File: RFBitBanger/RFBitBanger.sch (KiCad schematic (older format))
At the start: 174 parts, among them J1 POWER, J10 Conn_01x03, J11 SPEAKER, J12 Conn_Coaxial, J2 Barrel_Jack, J3 Conn_01x01, J4 Conn_01x01, J5 Conn_01x04, J6 Conn_01x01, J7 Conn_01x01, J9 ICSP, Q1 SS8050, Q2 SS9018, Q3 SS8050, Q4 S8050, Q5 SS8050, Q6 SS8050, Q7 SS8050, Q8 2N3906, Q9 SS8050, SW1 SW_Push, SW2 SW_Push, SW3 SW_Push, SW4 SW_Push, SW5 SW_Push, T1 Trifilar, T2 Trifilar, T3 Current, U1 ATMEGA328-PU, U2 LM7805_TO220, U3 LM386, U4 LM358, U5 LCD-016N002L, U6 SI5351A, Y1 16 MHz, Y2 7.023 MHz, Y3 27 MHz

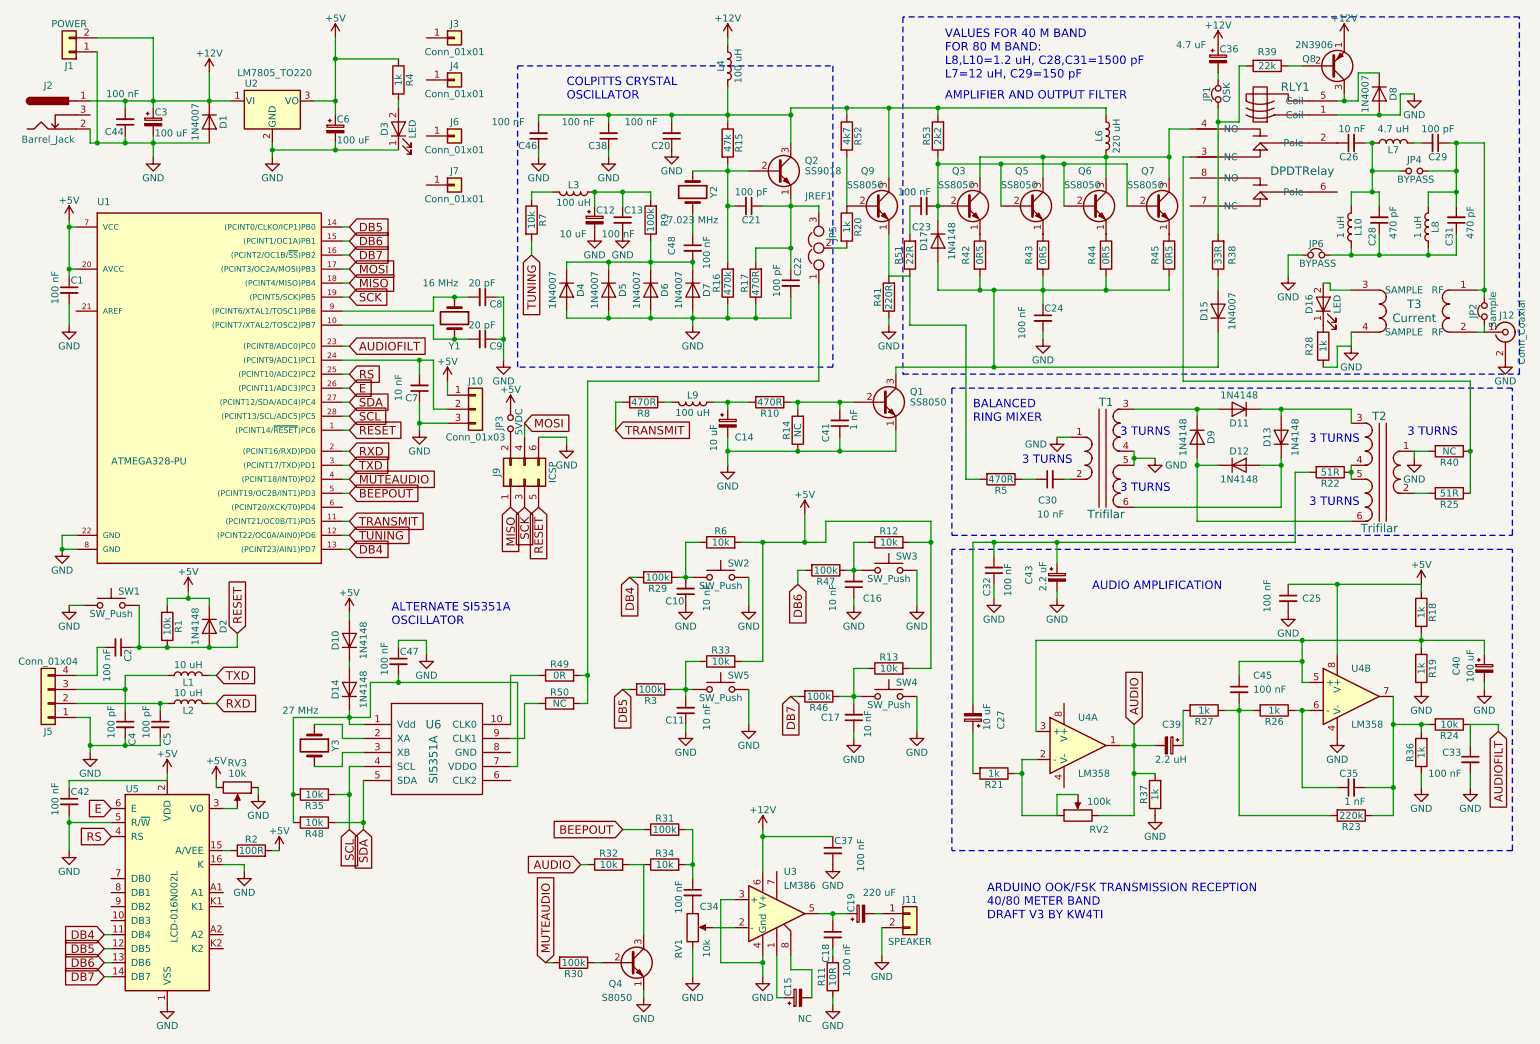
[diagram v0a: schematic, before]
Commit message: Completely remade board with common base input
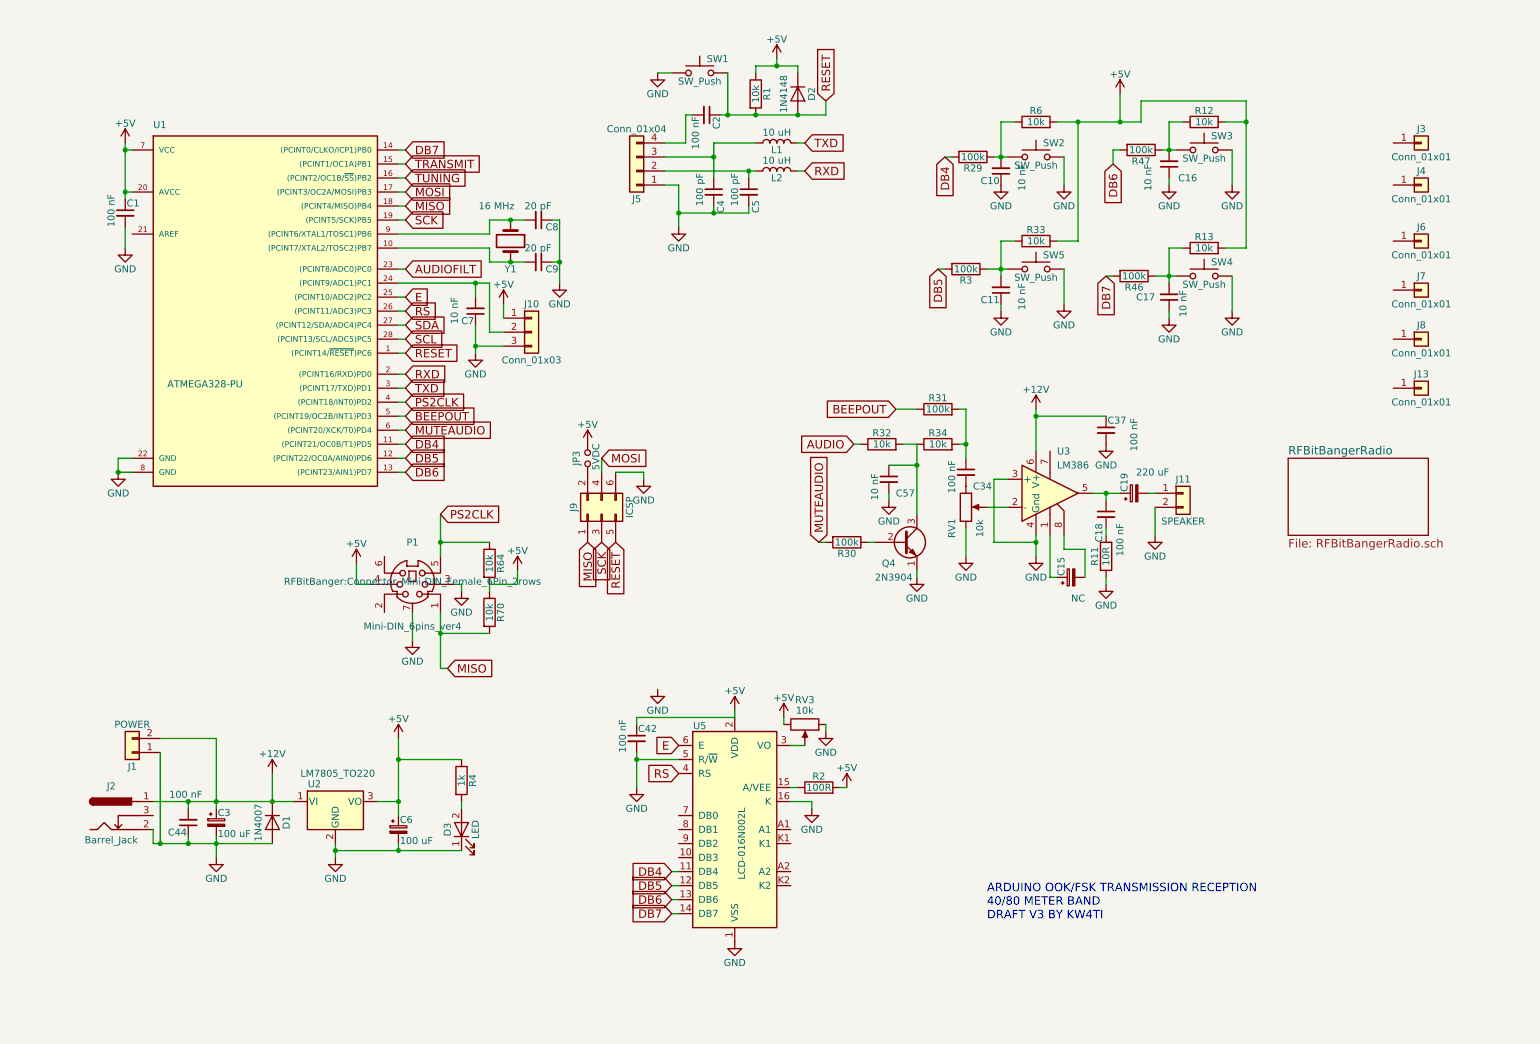
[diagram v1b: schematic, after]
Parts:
- removed C12, C14, C27: 10 uF, Capacitors_THT:CP_Radial_D5.0mm_P2.50mm, symbol CP_Small
- removed C13, C20, C23, C24, C25, C33, C38, C45, C46, C47, C48: 100 nF, Capacitors_THT:C_Disc_D5.0mm_W2.5mm_P2.50mm, symbol C_Small
- removed C21, C22, C29: 100 pF, Capacitors_THT:C_Disc_D5.0mm_W2.5mm_P5.00mm, symbol C_Small
- removed C26, C30: 10 nF, Capacitors_THT:C_Disc_D5.0mm_W2.5mm_P2.50mm, symbol C_Small
- removed C28, C31: 470 pF, Capacitors_THT:C_Disc_D5.0mm_W2.5mm_P5.00mm, symbol C_Small
- removed C32: 100 nF, Capacitors_THT:C_Disc_D5.0mm_W2.5mm_P5.00mm, symbol C_Small
- removed C35, C41: 1 nF, Capacitors_THT:C_Disc_D5.0mm_W2.5mm_P5.00mm, symbol C_Small
- removed C36: 4.7 uF, Capacitors_THT:CP_Radial_D5.0mm_P2.50mm, symbol CP_Small
- removed C39: 2.2 uH, Capacitors_THT:CP_Radial_D5.0mm_P2.50mm, symbol CP_Small
- removed C40: 100 uF, Capacitors_THT:CP_Radial_D5.0mm_P2.50mm, symbol CP_Small
- removed C43: 2.2 uF, Capacitors_THT:CP_Radial_D5.0mm_P2.50mm, symbol CP_Small
- removed D10, D11, D12, D13, D14, D17, D9: 1N4148, Diodes_THT:D_DO-35_SOD27_P7.62mm_Horizontal, symbol D
- removed D15, D4, D5, D6, D7, D8: 1N4007, Diodes_THT:D_DO-41_SOD81_P7.62mm_Horizontal, symbol D
- removed D16: LED, LEDs:LED_D3.0mm, symbol LED
- removed J12: Conn_Coaxial, RFBitBanger:bnc_90_1-1337543-0_pad_combo, symbol Conn_Coaxial
- removed JP1: QSK, Pin_Headers:Pin_Header_Straight_1x02_Pitch2.54mm, symbol Jumper_NC_Small
- removed JP2: Sample, Pin_Headers:Pin_Header_Straight_1x02_Pitch2.54mm, symbol Jumper_NC_Small
- removed JP4: BYPASS, Pin_Headers:Pin_Header_Straight_1x02_Pitch2.54mm, symbol Jumper_NO_Small
- removed JP5: JREF1, Pin_Headers:Pin_Header_Straight_1x03_Pitch2.54mm, symbol Jumper_NC_Dual
- removed JP6: BYPASS, Pin_Headers:Pin_Header_Straight_1x02_Pitch2.54mm, symbol Jumper_NC_Small
- removed L10, L8: 1 uH, Inductors_THT:L_Axial_L6.6mm_D2.7mm_P10.16mm_Horizontal_Vishay_IM-2, symbol L
- removed L3, L4, L9: 100 uH, Inductors_THT:L_Axial_L6.6mm_D2.7mm_P10.16mm_Horizontal_Vishay_IM-2, symbol L
- removed L6: 220 uH, Inductors_THT:L_Axial_L6.6mm_D2.7mm_P10.16mm_Horizontal_Vishay_IM-2, symbol L
- removed L7: 4.7 uH, Inductors_THT:L_Axial_L6.6mm_D2.7mm_P10.16mm_Horizontal_Vishay_IM-2, symbol L
- removed Q1, Q3, Q5, Q6, Q7, Q9: SS8050, TO_SOT_Packages_THT:TO-92_Inline_Wide, symbol 2N3904
- removed Q2: SS9018, TO_SOT_Packages_THT:TO-92_Inline_Wide, symbol 2N3904
- removed Q8: 2N3906, TO_SOT_Packages_THT:TO-92_Inline_Wide, symbol 2N3906
- removed R10, R17, R5, R8: 470R, Resistors_THT:R_Axial_DIN0207_L6.3mm_D2.5mm_P7.62mm_Horizontal, symbol R
- removed R14, R40, R50: NC, Resistors_THT:R_Axial_DIN0207_L6.3mm_D2.5mm_P7.62mm_Horizontal, symbol R
- removed R15: 47k, Resistors_THT:R_Axial_DIN0207_L6.3mm_D2.5mm_P7.62mm_Horizontal, symbol R
- removed R16: 470k, Resistors_THT:R_Axial_DIN0207_L6.3mm_D2.5mm_P7.62mm_Horizontal, symbol R
- removed R18, R19, R20, R21, R26, R27, R28, R36, R37: 1k, Resistors_THT:R_Axial_DIN0207_L6.3mm_D2.5mm_P7.62mm_Horizontal, symbol R
- removed R22, R25: 51R, Resistors_THT:R_Axial_DIN0207_L6.3mm_D2.5mm_P7.62mm_Horizontal, symbol R
- removed R23: 220k, Resistors_THT:R_Axial_DIN0207_L6.3mm_D2.5mm_P7.62mm_Horizontal, symbol R
- removed R24, R35, R48, R7: 10k, Resistors_THT:R_Axial_DIN0207_L6.3mm_D2.5mm_P7.62mm_Horizontal, symbol R
- removed R38: 33R, Resistors_THT:R_Axial_DIN0207_L6.3mm_D2.5mm_P7.62mm_Horizontal, symbol R
- removed R39: 22k, Resistors_THT:R_Axial_DIN0207_L6.3mm_D2.5mm_P7.62mm_Horizontal, symbol R
- removed R41: 220R, Resistors_THT:R_Axial_DIN0207_L6.3mm_D2.5mm_P7.62mm_Horizontal, symbol R
- removed R42, R43, R44, R45: 0R5, Resistors_THT:R_Axial_DIN0207_L6.3mm_D2.5mm_P7.62mm_Horizontal, symbol R
- removed R49: 0R, Resistors_THT:R_Axial_DIN0207_L6.3mm_D2.5mm_P7.62mm_Horizontal, symbol R
- removed R51: 22R, Resistors_THT:R_Axial_DIN0207_L6.3mm_D2.5mm_P7.62mm_Horizontal, symbol R
- removed R52: 4k7, Resistors_THT:R_Axial_DIN0207_L6.3mm_D2.5mm_P7.62mm_Horizontal, symbol R
- removed R53: 2k2, Resistors_THT:R_Axial_DIN0207_L6.3mm_D2.5mm_P7.62mm_Horizontal, symbol R
- removed R9: 100k, Resistors_THT:R_Axial_DIN0207_L6.3mm_D2.5mm_P7.62mm_Horizontal, symbol R
- removed RLY1: DPDTRelay, RFBitBanger:G2VRelay, symbol DPDTRelay
- removed RV2: 100k, Potentiometers:Potentiometer_WirePads, symbol POT
- removed T1, T2: Trifilar, RFBitBanger:TripleWindingTransformer, symbol TripleWindingTransformer
- removed T3: Current, RFBitBanger:SamplingTransformer, symbol Current
- removed U4: LM358, Housings_DIP:DIP-8_W7.62mm_Socket, symbol LM358
- removed U6: SI5351A, Housings_SSOP:MSOP-10_3x3mm_Pitch0.5mm, symbol SI5351A
- removed Y2: 7.023 MHz, Crystals:Crystal_HC49-U_Vertical, symbol Crystal
- removed Y3: 27 MHz, Crystals:Crystal_HC49-U_Vertical, symbol Crystal
- added C57: 10 nF, Capacitors_THT:C_Disc_D5.0mm_W2.5mm_P2.50mm, symbol C_Small
- added J13, J8: Conn_01x01, Connectors:1pin, symbol Conn_01x01
- added P1: Mini-DIN_6pins_ver4, RFBitBanger:Connector_Mini-DIN_Female_6Pin_2rows, symbol Mini-DIN_6pins_ver4
- added R64, R70: 10k, Resistors_THT:R_Axial_DIN0207_L6.3mm_D2.5mm_P7.62mm_Horizontal, symbol R
- Q4: value S8050 -> 2N3904
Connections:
- net +5V: now also P1.4, R64.2, R70.1
- net DB4: now also U1.11 ((PCINT21/OC0B/T1)PD5); no longer U1.13 ((PCINT23/AIN1)PD7)
- net DB5: now also U1.12 ((PCINT22/OC0A/AIN0)PD6); no longer U1.14 ((PCINT0/CLKO/ICP1)PB0)
- net DB6: now also U1.13 ((PCINT23/AIN1)PD7); no longer U1.15 ((PCINT1/OC1A)PB1)
- net DB7: now also U1.14 ((PCINT0/CLKO/ICP1)PB0); no longer U1.16 ((PCINT2/OC1B/~SS~)PB2)
- net E: now also U1.25 ((PCINT10/ADC2)PC2); no longer U1.26 ((PCINT11/ADC3)PC3)
- net GND: now also C57.2, P1.3, P1.7 (Shell)
- net MISO: now also P1.1, R70.2
- net MUTEAUDIO: now also U1.6 ((PCINT20/XCK/T0)PD4); no longer U1.4 ((PCINT18/INT0)PD2)
- net RS: now also U1.26 ((PCINT11/ADC3)PC3); no longer U1.25 ((PCINT10/ADC2)PC2)
- net TRANSMIT: now also U1.15 ((PCINT1/OC1A)PB1); no longer U1.11 ((PCINT21/OC0B/T1)PD5)
- net TUNING: now also U1.16 ((PCINT2/OC1B/~SS~)PB2); no longer U1.12 ((PCINT22/OC0A/AIN0)PD6)
- net at Q4.3 (C), R32.2, R34.1: now also C57.1
- new net PS2CLK: P1.5, R64.1, U1.4 ((PCINT18/INT0)PD2)
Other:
- note removed: "3 TURNS"
- note removed: "3 TURNS\n"
- note removed: "ALTERNATE SI5351A\nOSCILLATOR"
- note removed: "AMPLIFIER AND OUTPUT FILTER"
- note removed: "AUDIO AMPLIFICATION"
- note removed: "BALANCED\nRING MIXER"
- note removed: "COLPITTS CRYSTAL\nOSCILLATOR"
- note removed: "VALUES FOR 40 M BAND\nFOR 80 M BAND:\nL8,L10=1.2 uH, C28,C31=1500 pF\nL7=12 uH, C29=150 pF"
- moved on the sheet: C1, C10, C11, C15, C16, C17, C18, C19, C2, C3, C34, C37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
